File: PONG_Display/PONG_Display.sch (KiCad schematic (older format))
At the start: 8 parts

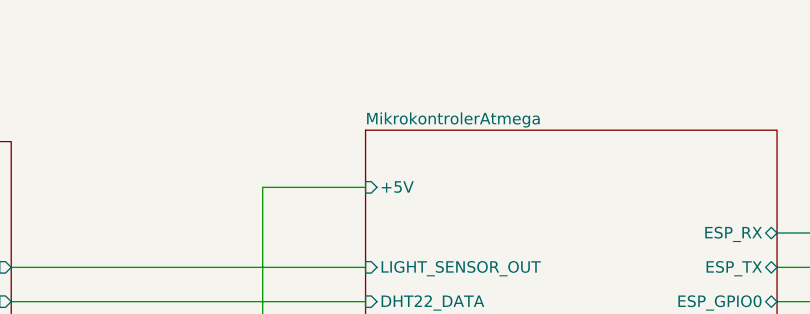
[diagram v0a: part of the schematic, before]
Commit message: test brancha
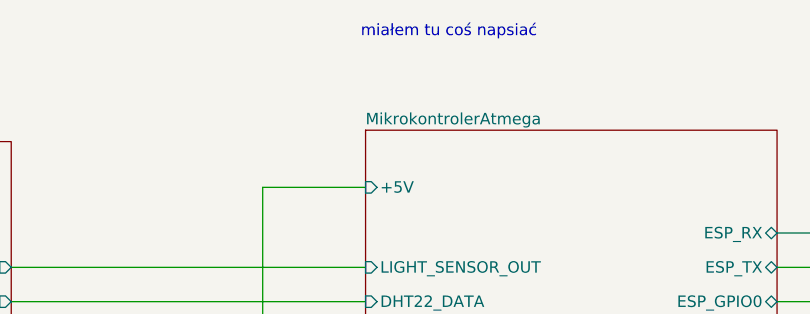
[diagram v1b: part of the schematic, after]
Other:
- note added: "miałem tu coś napsiać\n"
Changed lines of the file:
@@
 EESchema Schematic File Version 4
+LIBS:PONG_Display-cache
 EELAYER 30 0
 EELAYER END
@@
 Text Notes 7600 7500 0    50   ~ 0
 Wyświetlacz ping-pong - schemat główny
+Text Notes 6150 1500 2    50   ~ 0
+miałem tu coś napsiać\n
 $EndSCHEMATC

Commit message: nowe
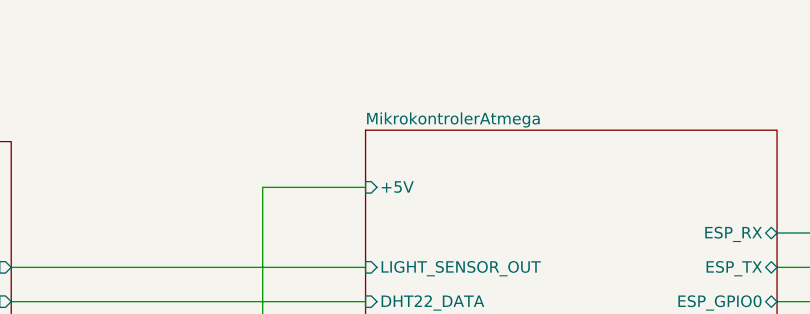
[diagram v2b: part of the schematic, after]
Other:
- note removed: "miałem tu coś napsiać\n"
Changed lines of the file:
@@
 EESchema Schematic File Version 4
-LIBS:PONG_Display-cache
 EELAYER 30 0
 EELAYER END
@@
 Text Notes 7600 7500 0    50   ~ 0
 Wyświetlacz ping-pong - schemat główny
-Text Notes 6150 1500 2    50   ~ 0
-miałem tu coś napsiać\n
 $EndSCHEMATC
